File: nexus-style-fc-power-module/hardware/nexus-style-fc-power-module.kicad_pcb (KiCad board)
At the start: 4 copper layers, 26 x 22 mm, 30 parts, among them J1 PWR IN, J2 PWR OUT, U14 TPS629210DRLR, U5 TPS62130RGTR, U9 TPS2116DRLR

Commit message: added standalone power module
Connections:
- net 5V_BUCK renamed /5V_BUCK
- net FB_5V renamed /FB_5V
- net PR1 renamed /PR1
- net SCONF renamed /SCONF
- net SS_5V renamed /SS_5V
- net SW_3V3 renamed /SW_3V3
- net SW_5V renamed /SW_5V

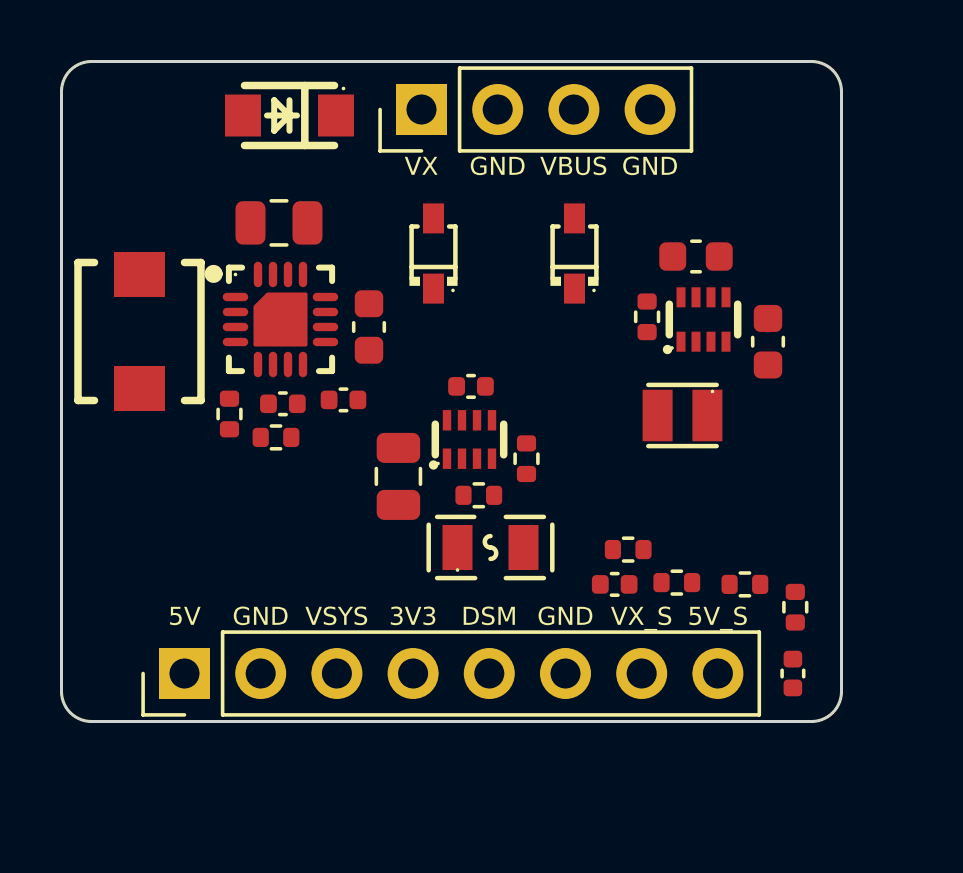
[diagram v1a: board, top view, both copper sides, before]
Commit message: added usbc
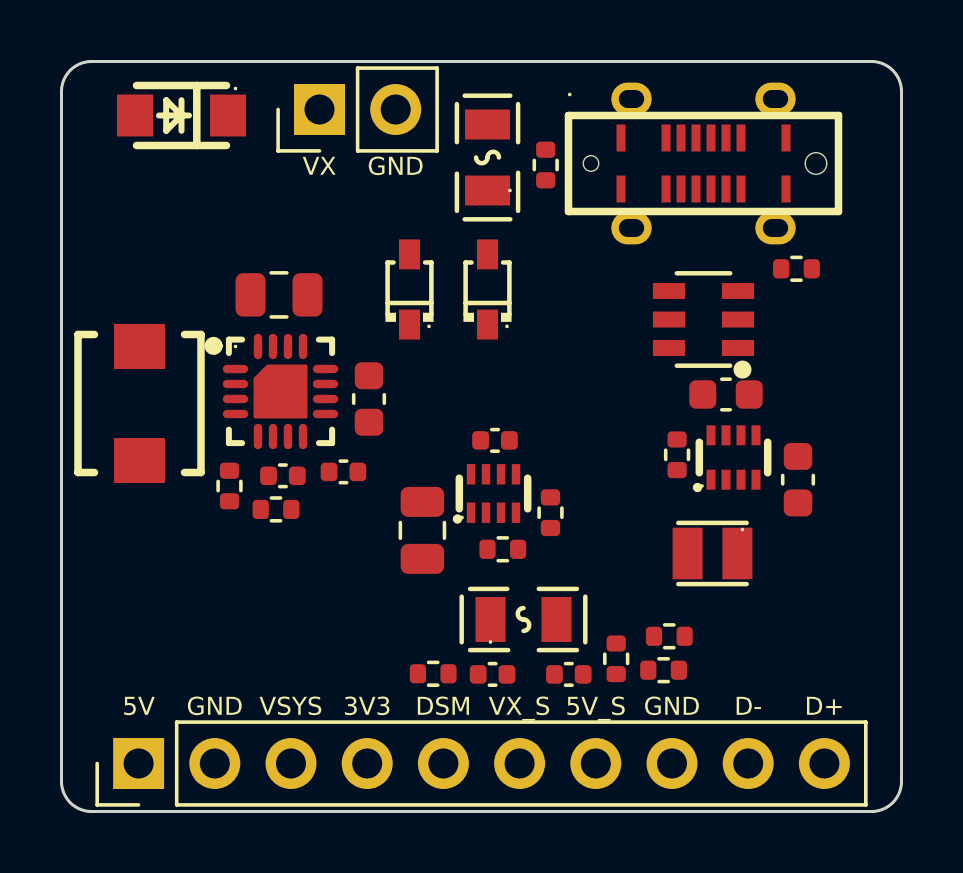
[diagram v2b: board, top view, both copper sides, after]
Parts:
- added F1: 0.5A PTC, NexusFC:F0805, F.Cu at (114.2, 103.2)
- added J6: USB-C vertical, NexusFC:USB-C-SMD_TYPE-C-31-D-06, F.Cu at (121.4, 103.4)
- added R20: 5.1k, Resistor_SMD:R_0402_1005Metric, F.Cu at (116.1, 103.5)
- added R21: 5.1k, Resistor_SMD:R_0402_1005Metric, F.Cu at (124.5, 106.9)
- added U7: USBLC6-2SC6, NexusFC:SOT-23-6_L2.9-W1.6-P0.95-LS2.8-BL, F.Cu at (121.4, 108.6)
- J1: footprint Connector_PinHeader_2.54mm:PinHeader_1x04_P2.54mm_Vertical -> Connector_PinHeader_2.54mm:PinHeader_1x02_P2.54mm_Vertical
- J2: footprint Connector_PinHeader_2.54mm:PinHeader_1x08_P2.54mm_Vertical -> Connector_PinHeader_2.54mm:PinHeader_1x10_P2.54mm_Vertical
- moved R16 8.67 mm to (112.4, 120.4)
- moved C30 7.47 mm to (116.9, 120.4), turned to 0 degrees
- moved C29 5.06 mm to (114.4, 120.4)
- moved L2 4.71 mm to (121.7, 116.4)
- moved U14 4.71 mm to (122.4, 113.2)
- moved C27 4.71 mm to (122.2, 111.1)
- moved C28 4.71 mm to (124.5, 113.9)
- moved R15 4.71 mm to (120.5, 113.1)
- moved R19 4.31 mm to (120.3, 119.2), turned to 0 degrees
- moved R18 3.94 mm to (120.1, 120.3)
- moved R17 3.66 mm to (118.5, 119.9), turned to 90 degrees
- moved D4 3.60 mm to (104.0, 101.8)
- moved J1 3.40 mm to (108.6, 101.6)
- moved J2 3.37 mm to (102.6, 123.4)
- moved D6 3.14 mm to (114.2, 107.6)
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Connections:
- J2 pad 6: GND -> VX_SENSE
- J2 pad 7: VX_SENSE -> 5V_SENSE
- J2 pad 8: 5V_SENSE -> GND
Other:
- board size 26 x 22 mm -> 28 x 25 mm
- board text added: "D+"
- board text added: "D-"
- board text added: "Nexus-style FC power module 28.0 x 25.0 mm, rev 0.1"
- board text removed: "Nexus-style FC power module 26.0 x 22.0 mm, rev 0.1"
- board text removed: "VBUS"
